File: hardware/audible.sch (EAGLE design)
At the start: 27 parts, among them IC1 LTC1966CMS8, J1 SQUALL_HEADER, J2 HIROSE-DF40C-10DP-0.4V, J3 HIROSE-DF40C-10DP-0.4V, J5 TC2030-JLINK-NL, Q1 FK3503010L, U1 MAX417ESA+, U2 MAX417ESA+

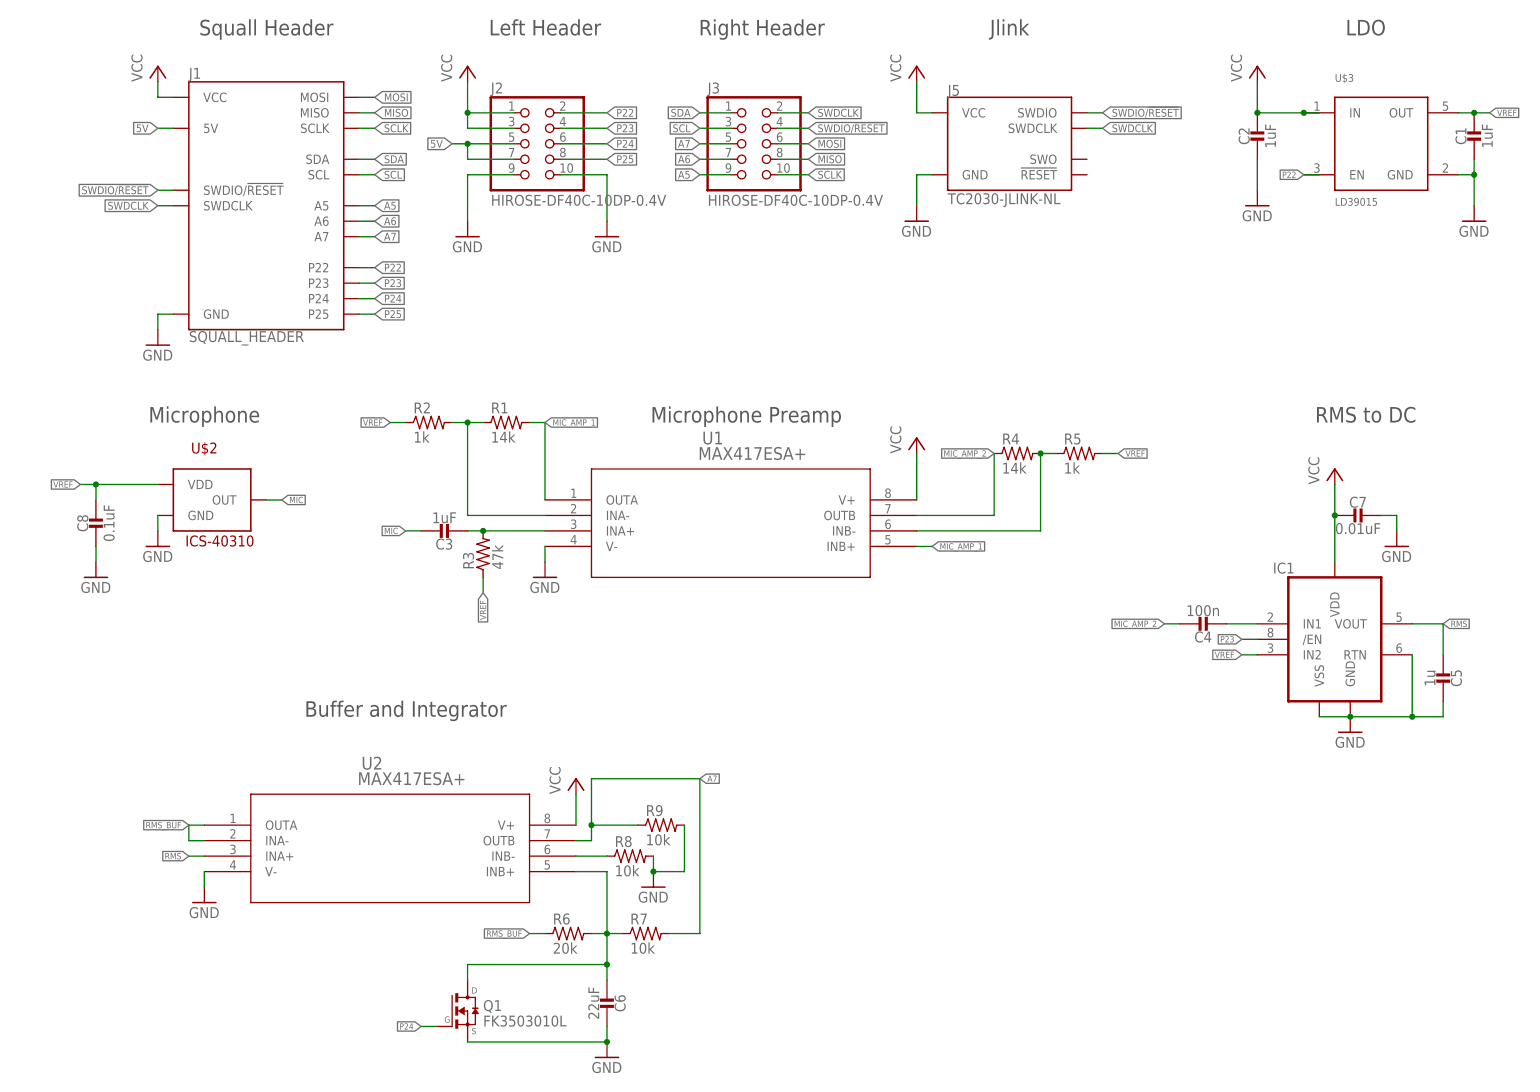
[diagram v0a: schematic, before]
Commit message: Updated sch and brd
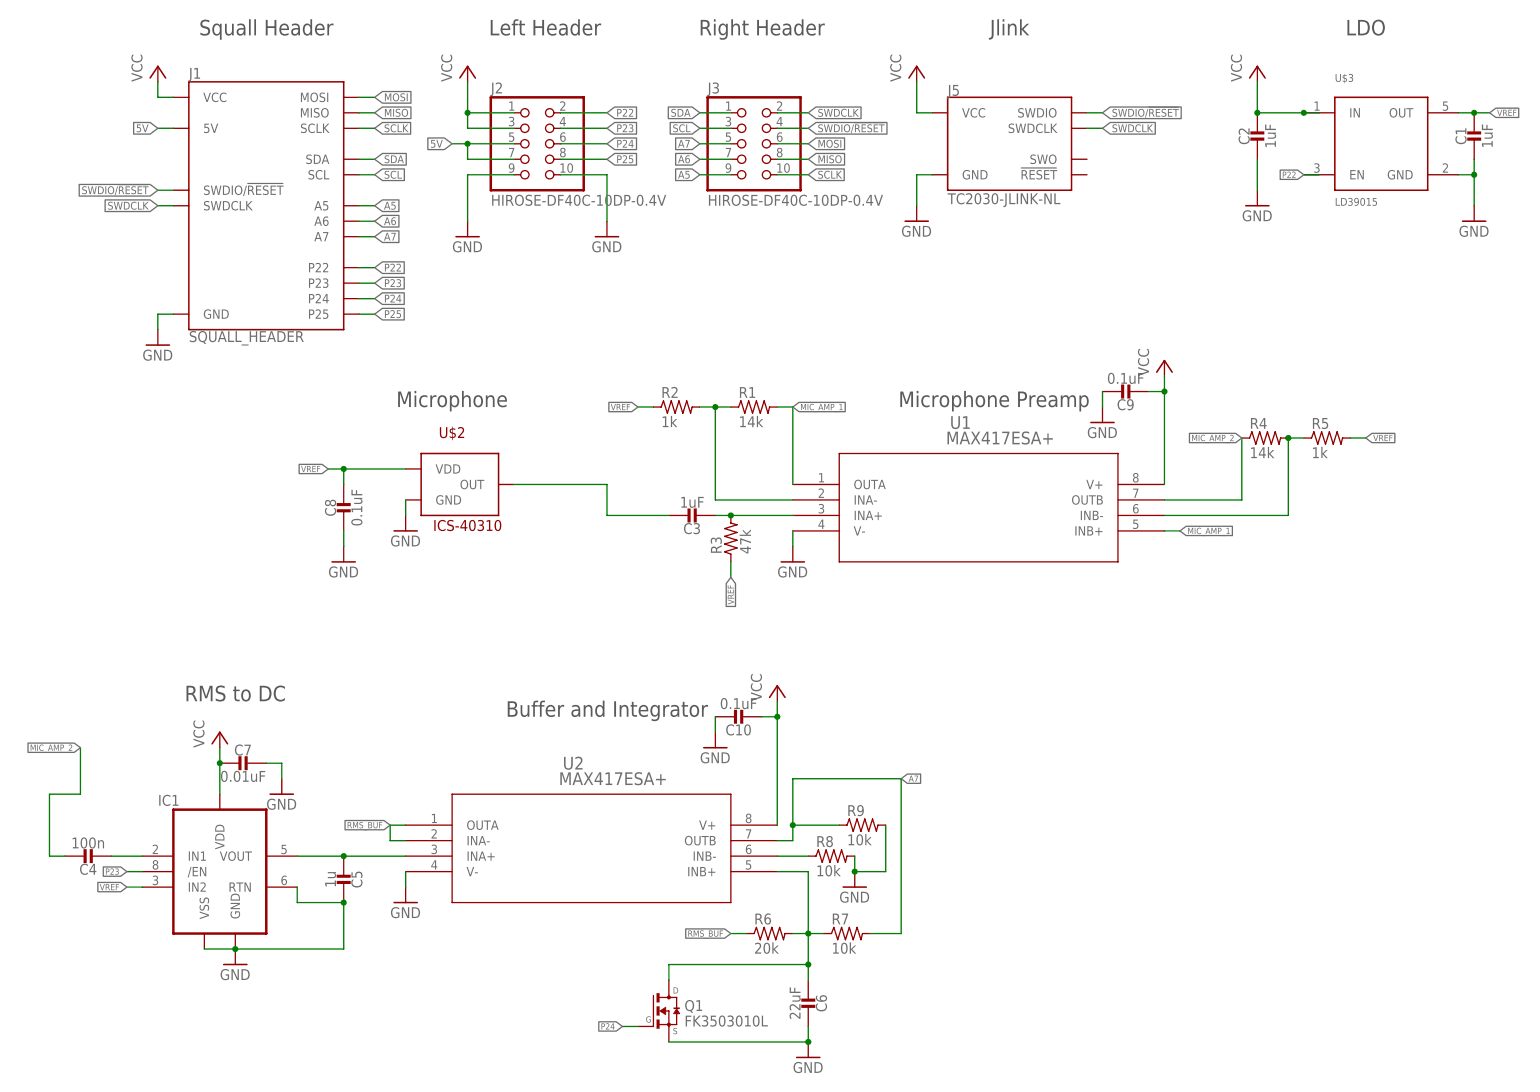
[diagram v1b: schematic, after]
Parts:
- added C10, C9: 0.1uF, passives:CAPACITOR
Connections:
- net RMS renamed N$3
- net GND: now also C10.1, C9.1
- net VCC: now also C10.2, C9.2
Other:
- moved on the sheet: C3, C4, C5, C6, C7, C8, IC1, Q1, R1, R2, R3, R4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
